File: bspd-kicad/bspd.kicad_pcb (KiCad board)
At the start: 4 copper layers, 79.5 x 60.8 mm, 114 parts, among them J1 BSPD Connector, Q1 AO3400A, Q2 AO3401A, SW1 CJS-1200TB1, SW2 CJS-1200TB1, U5 SN74HC74DR, U6 LM1117MP-5.0, U7 SN74LVC2G14DBVR, U8 SN74LVC3G14DCUR, U9 SN74LVC3G14DCUR

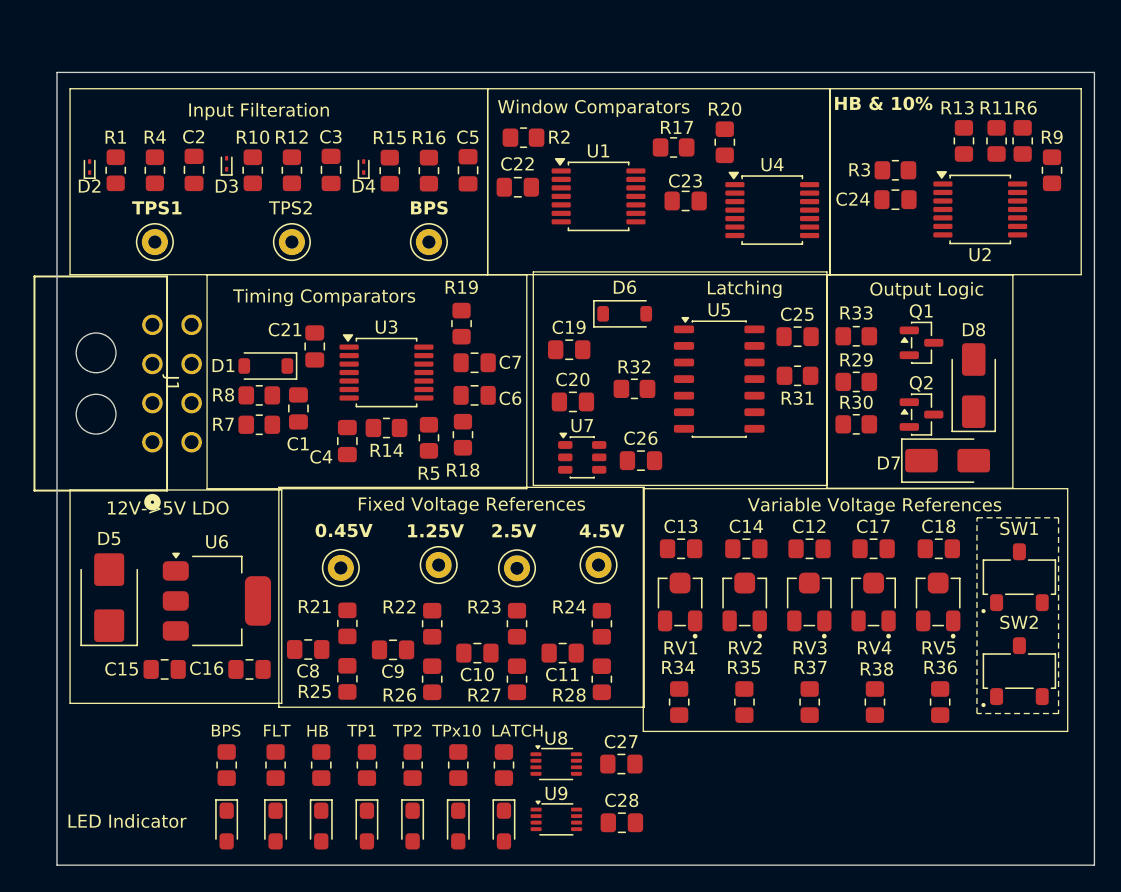
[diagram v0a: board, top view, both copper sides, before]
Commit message: Draft complete
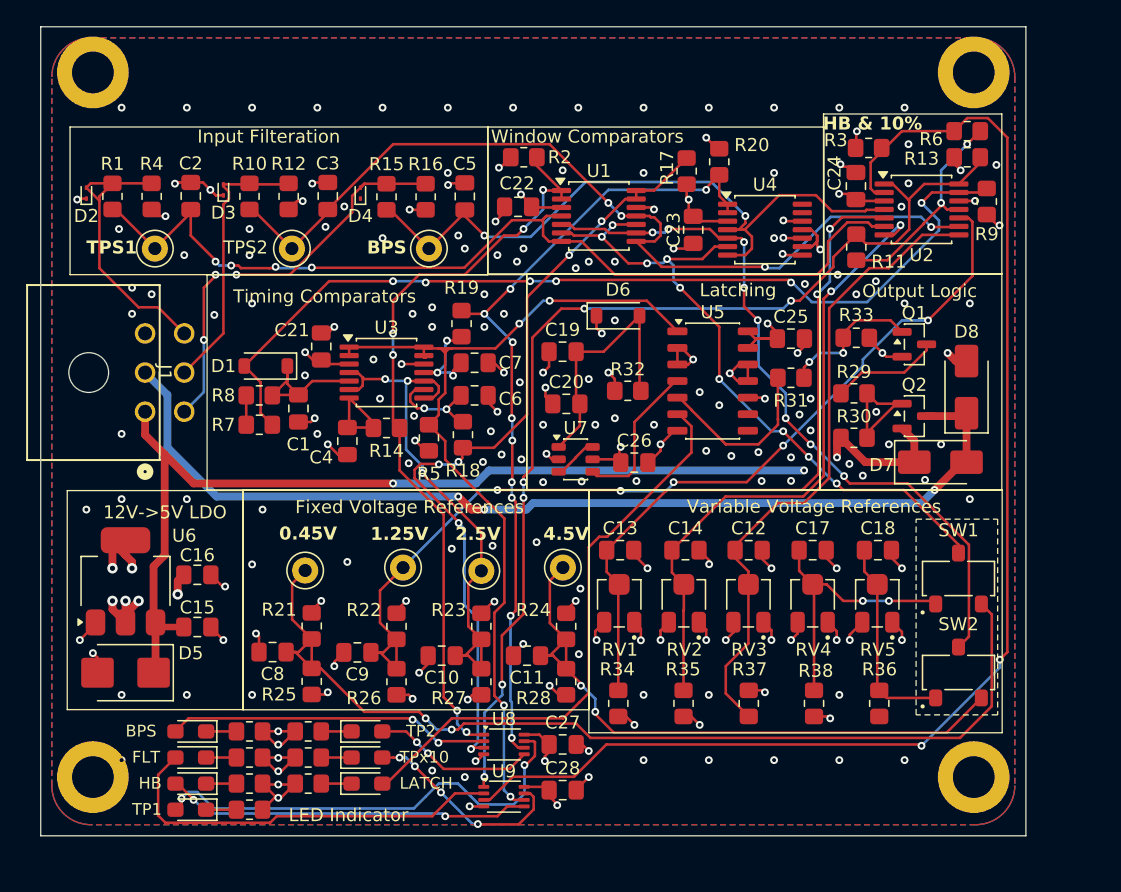
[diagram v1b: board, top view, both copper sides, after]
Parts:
- added H1: MountingHole_Pad, MountingHole:MountingHole_3.2mm_M3_ISO14580_Pad, F.Cu at (95.0, 97.0)
- added H2: MountingHole_Pad, MountingHole:MountingHole_3.2mm_M3_ISO14580_Pad, F.Cu at (27.5, 151.0)
- added H3: MountingHole_Pad, MountingHole:MountingHole_3.2mm_M3_ISO14580_Pad, F.Cu at (27.5, 97.0)
- added H4: MountingHole_Pad, MountingHole:MountingHole_3.2mm_M3_ISO14580_Pad, F.Cu at (95.0, 151.0)
- J1: footprint bspd:MOLEX_430450800 -> bspd:MOLEX_430450600
- R29: value 47k -> 49.9k
- R30: value 56k -> 54.9k
- moved R39 15.1 mm to (44.0, 151.5), turned to 180 degrees
- moved D10 13.6 mm to (35.0, 153.5), turned to 180 degrees
- moved R11 13.5 mm to (86.0, 110.4), turned to 90 degrees
- moved R41 11.5 mm to (44.0, 149.5), turned to 180 degrees
- moved D9 11.0 mm to (48.5, 151.5), turned to 0 degrees
- moved D13 10.5 mm to (35.0, 151.5), turned to 180 degrees
- moved R40 9.63 mm to (39.5, 153.5), turned to 0 degrees
- moved D11 8.75 mm to (48.5, 149.5), turned to 0 degrees
- moved R42 8.41 mm to (44.0, 147.5), turned to 180 degrees
- moved D14 8.36 mm to (35.0, 149.5), turned to 180 degrees
- moved C16 8.28 mm to (35.5, 135.5), turned to 180 degrees
- moved D12 8.05 mm to (48.5, 147.5), turned to 0 degrees
- moved D15 7.76 mm to (35.0, 147.5), turned to 180 degrees
- moved U6 7.16 mm to (30.0, 136.0), turned to 90 degrees
- moved D5 5.88 mm to (30.0, 143.0), turned to 180 degrees
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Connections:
- R30 pad 1: Net-(Q2-G) -> +12V
- R30 pad 2: +12V -> Net-(Q2-G)
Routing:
- net Earth: track 0.00 -> 117.3 mm, vias 0 -> 183
- net HB: track 0.00 -> 100.4 mm, vias 0 -> 2
- net +12V: track 0.00 -> 87.7 mm, vias 0 -> 3
- net TPSx10%: track 0.00 -> 81.1 mm, vias 0 -> 6
- net +5V: track 0.00 -> 80.8 mm, vias 0 -> 35
- net SC_OUT: track 0.00 -> 78.1 mm, vias 0 -> 3
- net +0V45: track 0.00 -> 77.3 mm, vias 0 -> 2
- net TPS1: track 0.00 -> 73.9 mm, vias 0 -> 4
- net HB&10%: track 0.00 -> 72.8 mm, vias 0 -> 6
- net +1V25: track 0.00 -> 72.6 mm, vias 0 -> 5
- net FAULT: track 0.00 -> 70.1 mm, vias 0 -> 4
- net TPS2: track 0.00 -> 69.3 mm, vias 0 -> 4
- net BPS_FAULT: track 0.00 -> 63.3 mm, vias 0 -> 10
- net TPS2_FAULT: track 0.00 -> 61.9 mm, vias 0 -> 6
- net TPS1_FAULT: track 0.00 -> 58.2 mm, vias 0 -> 6
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- added copper zone on In2.Cu, net +5V
- added copper zone on B.Cu, net Earth
- added copper zone on F.Cu, net Earth
- added copper zone on In1.Cu, net Earth
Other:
- board size 79.5 x 60.8 mm -> 75.5 x 62 mm
